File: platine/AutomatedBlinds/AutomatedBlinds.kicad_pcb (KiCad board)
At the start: 2 copper layers, 17.8 x 43.2 mm, 6 parts, among them P1 Digital, P2 Analog, P3 CONN_01X01, P4 CONN_01X01, P5 CONN_01X01, P6 CONN_01X01

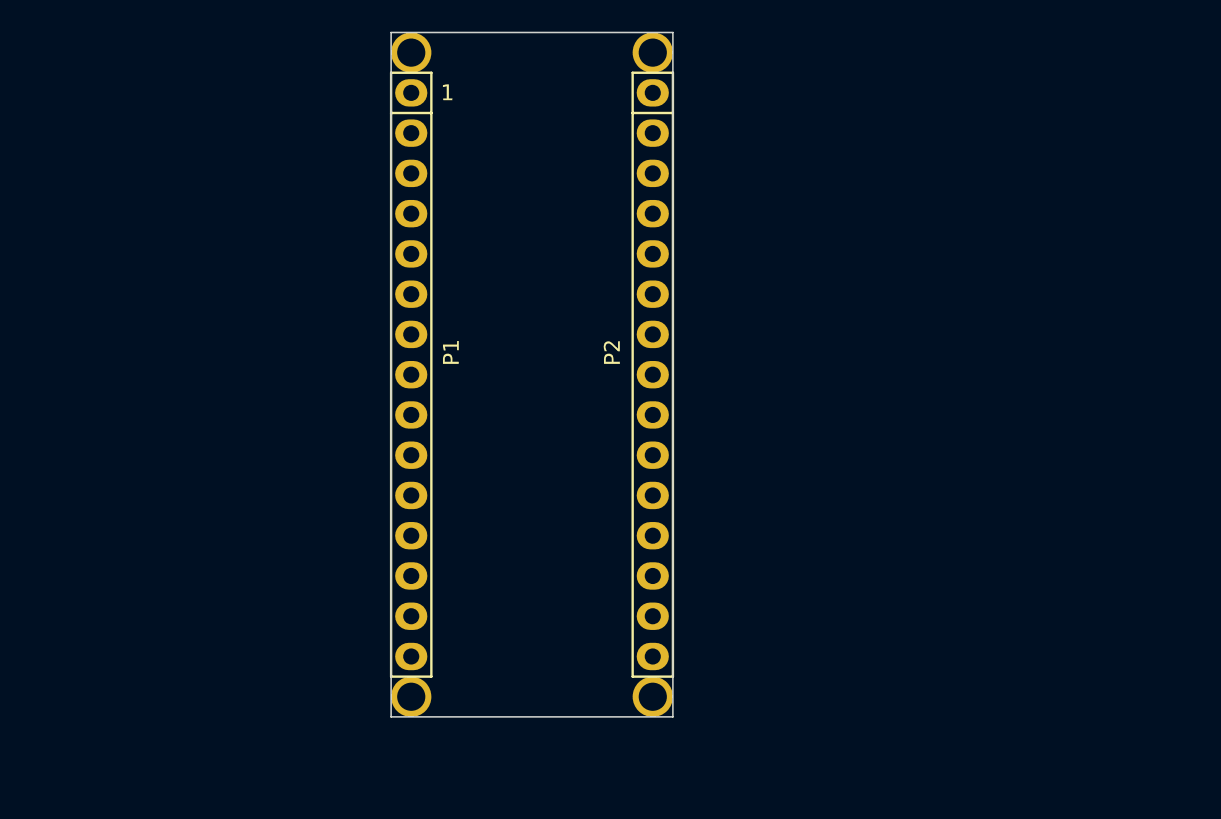
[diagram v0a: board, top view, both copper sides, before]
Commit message: minor
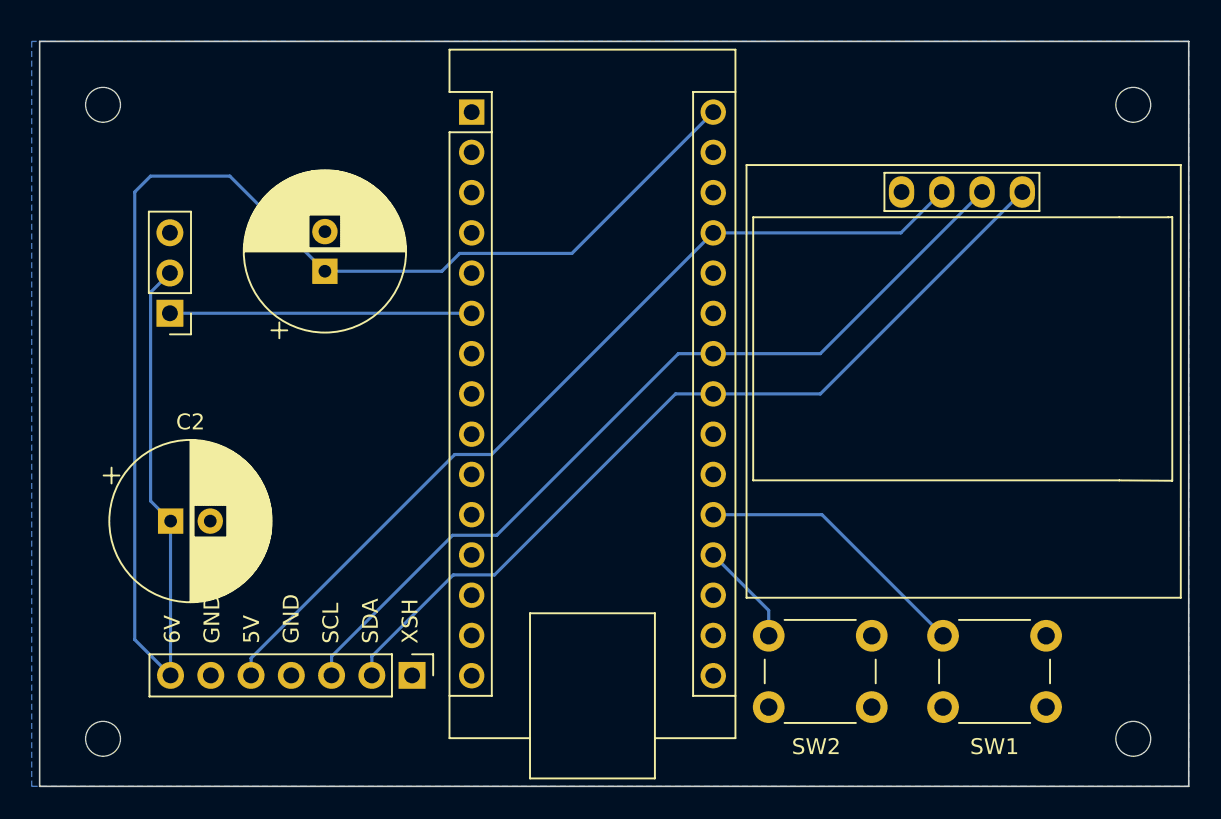
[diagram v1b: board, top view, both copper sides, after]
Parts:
- removed P1: Digital, Socket_Arduino_Nano:Socket_Strip_Arduino_1x15
- removed P2: Analog, Socket_Arduino_Nano:Socket_Strip_Arduino_1x15
- removed P3, P4, P5, P6: CONN_01X01, Socket_Arduino_Nano:1pin_Nano
- added A1: Arduino_Nano_v3.x, Module:Arduino_Nano, F.Cu at (143.3, 72.5)
- added Brd1: SSD1306, SSD1305:128x64OLED, F.Cu at (174.0, 88.1)
- added C1: C, Capacitor_THT:CP_Radial_D10.0mm_P2.50mm, F.Cu at (134.0, 82.5)
- added C2: C, Capacitor_THT:CP_Radial_D10.0mm_P2.50mm, F.Cu at (124.3, 98.3)
- added H1: MountingHole, MountingHole:MountingHole_2.2mm_M2, F.Cu at (120.0, 72.0)
- added H2: MountingHole, MountingHole:MountingHole_2.2mm_M2, F.Cu at (185.0, 72.0)
- added H3: MountingHole, MountingHole:MountingHole_2.2mm_M2, F.Cu at (185.0, 112.0)
- added H4: MountingHole, MountingHole:MountingHole_2.2mm_M2, F.Cu at (120.0, 112.0)
- added J2: Conn_01x03_Male, Connector_PinHeader_2.54mm:PinHeader_1x03_P2.54mm_Vertical, F.Cu at (124.2, 85.2)
- added J4: Conn_01x07_Male, Connector_PinHeader_2.54mm:PinHeader_1x07_P2.54mm_Vertical, F.Cu at (139.5, 108.0)
- added SW1: SW_Push, Button_Switch_THT:SW_PUSH_6mm_H4.3mm, F.Cu at (173.0, 105.5)
- added SW2: SW_Push, Button_Switch_THT:SW_PUSH_6mm_H4.3mm, F.Cu at (162.0, 105.5)
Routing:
- net +6V: track 0.00 -> 101.6 mm
- net +5V: track 0.00 -> 57.2 mm
- net Net-(A1-A5): track 0.00 -> 54.4 mm
- net Net-(A1-A4): track 0.00 -> 54.4 mm
- net Net-(A1-D3): track 0.00 -> 19.0 mm
- net Net-(A1-A1): track 0.00 -> 17.7 mm
- net Net-(A1-A0): track 0.00 -> 6.95 mm
- added copper zone on B.Cu, net GND
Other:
- board size 17.8 x 43.2 mm -> 72.5 x 47 mm
- net class Default removed
- board text added: "5V"
- board text added: "6V"
- board text added: "GND"
- board text added: "SCL"
- board text added: "SDA"
- board text added: "XSH"
- board text removed: "1"
